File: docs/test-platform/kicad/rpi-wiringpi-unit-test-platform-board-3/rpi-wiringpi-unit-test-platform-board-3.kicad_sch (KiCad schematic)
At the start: 22 parts, among them J1 JST_IN_PWR, J2 JST_IN_SIG, J3 JST_OUT_PWR, J4 JST_OUT_SW, J5 JST_OUT_COIL, J6 JST_IO_A4_7, J7 JST_IO_B0_3, J8 JST_IO_B4_7, SW1 DIP_SW_x3, U1 MCP23017_0x20, U2 MCP23017_0x21

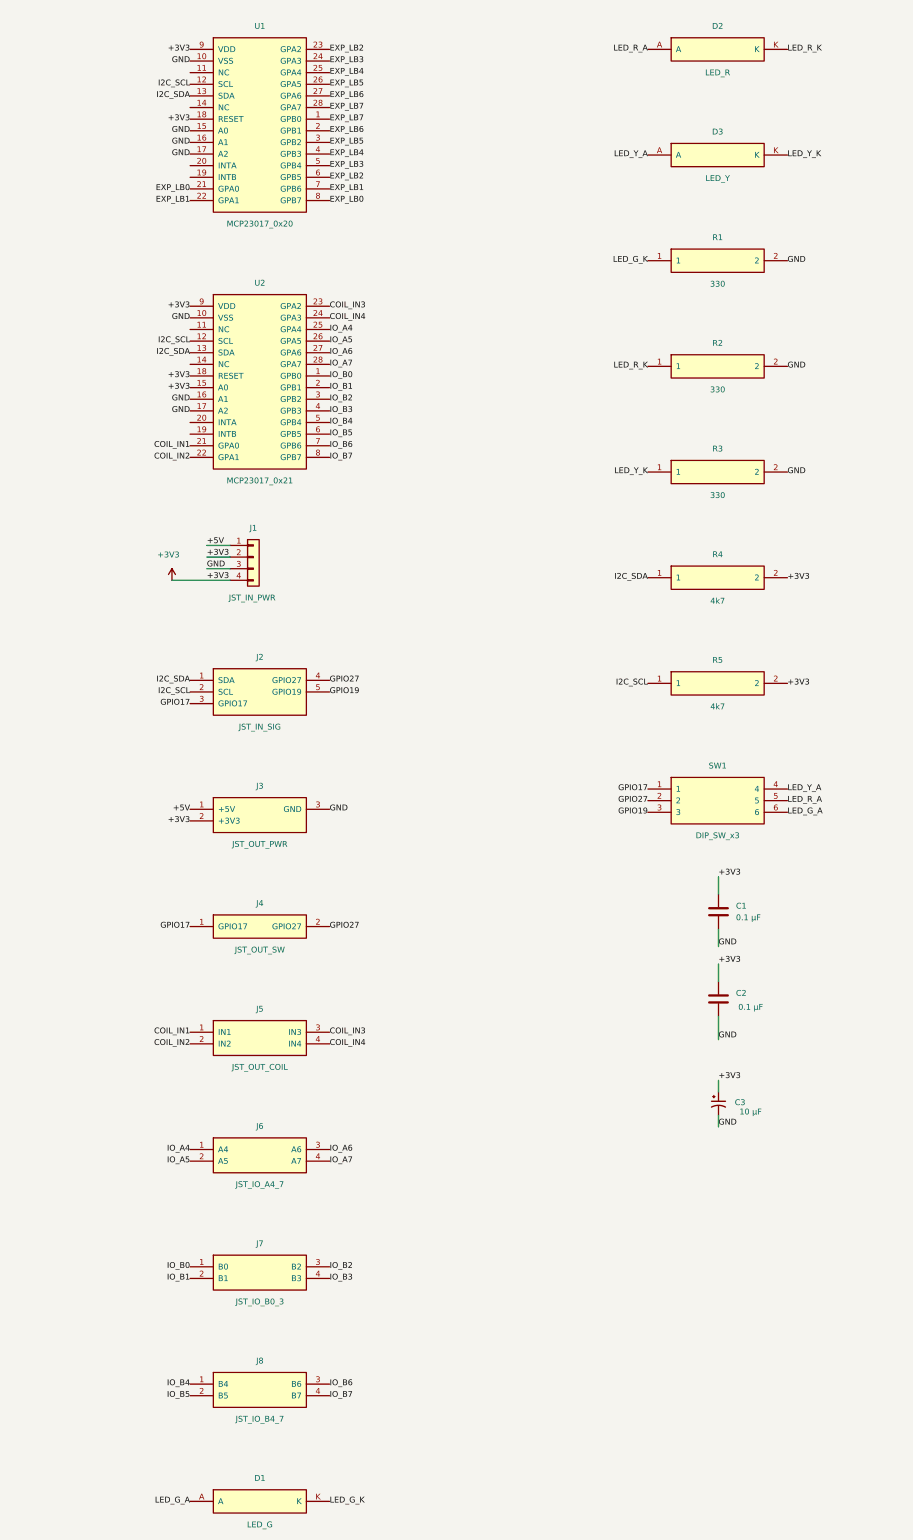
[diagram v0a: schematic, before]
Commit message: Updated boards
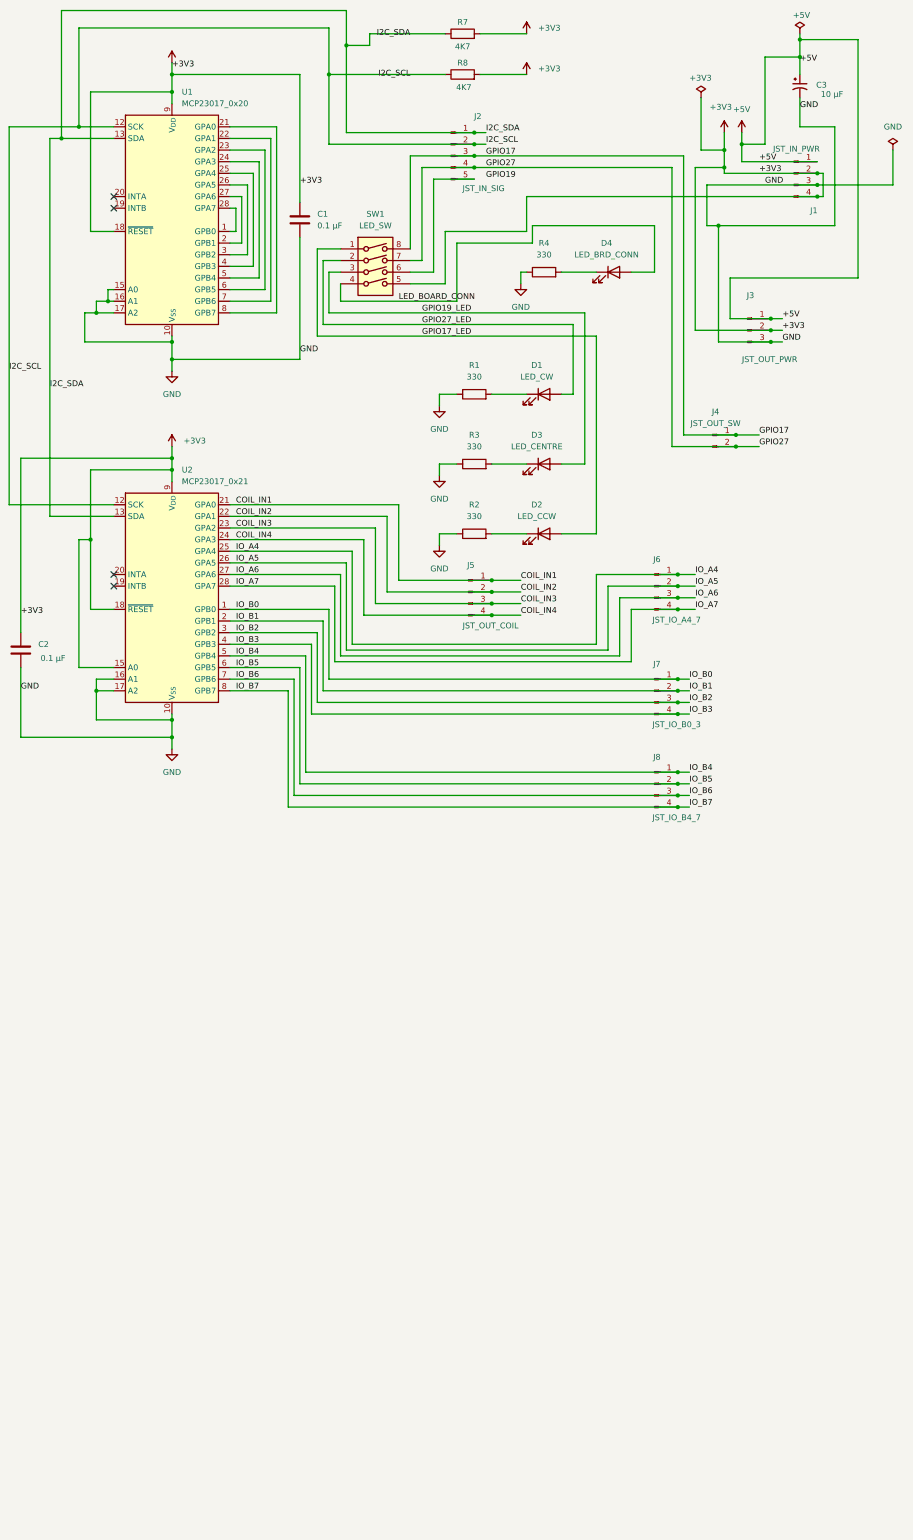
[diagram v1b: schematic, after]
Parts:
- removed D1: LED_G, rpi-wiringpi-unit-test-platform-board-3:D1, symbol rpi-wiringpi-unit-test-platform-board-3:D1
- removed D2: LED_R, rpi-wiringpi-unit-test-platform-board-3:D2, symbol rpi-wiringpi-unit-test-platform-board-3:D2
- removed D3: LED_Y, rpi-wiringpi-unit-test-platform-board-3:D3, symbol rpi-wiringpi-unit-test-platform-board-3:D3
- removed J1: JST_IN_PWR, rpi-wiringpi-unit-test-platform-board-3:J1, symbol Connector_Generic:Conn_01x04
- removed J2: JST_IN_SIG, rpi-wiringpi-unit-test-platform-board-3:J2, symbol rpi-wiringpi-unit-test-platform-board-3:J2
- removed J3: JST_OUT_PWR, rpi-wiringpi-unit-test-platform-board-3:J3, symbol rpi-wiringpi-unit-test-platform-board-3:J3
- removed J4: JST_OUT_SW, rpi-wiringpi-unit-test-platform-board-3:J4, symbol rpi-wiringpi-unit-test-platform-board-3:J4
- removed J5: JST_OUT_COIL, rpi-wiringpi-unit-test-platform-board-3:J5, symbol rpi-wiringpi-unit-test-platform-board-3:J5
- removed J6: JST_IO_A4_7, rpi-wiringpi-unit-test-platform-board-3:J6, symbol rpi-wiringpi-unit-test-platform-board-3:J6
- removed J7: JST_IO_B0_3, rpi-wiringpi-unit-test-platform-board-3:J7, symbol rpi-wiringpi-unit-test-platform-board-3:J7
- removed J8: JST_IO_B4_7, rpi-wiringpi-unit-test-platform-board-3:J8, symbol rpi-wiringpi-unit-test-platform-board-3:J8
- removed R1: 330, rpi-wiringpi-unit-test-platform-board-3:R1, symbol rpi-wiringpi-unit-test-platform-board-3:R1
- removed R2: 330, rpi-wiringpi-unit-test-platform-board-3:R2, symbol rpi-wiringpi-unit-test-platform-board-3:R2
- removed R3: 330, rpi-wiringpi-unit-test-platform-board-3:R3, symbol rpi-wiringpi-unit-test-platform-board-3:R3
- removed R4: 4k7, rpi-wiringpi-unit-test-platform-board-3:R4, symbol rpi-wiringpi-unit-test-platform-board-3:R4
- removed R5: 4k7, rpi-wiringpi-unit-test-platform-board-3:R5, symbol rpi-wiringpi-unit-test-platform-board-3:R5
- removed SW1: DIP_SW_x3, rpi-wiringpi-unit-test-platform-board-3:SW1, symbol rpi-wiringpi-unit-test-platform-board-3:SW1
- removed U1: MCP23017_0x20, rpi-wiringpi-unit-test-platform-board-3:U1, symbol rpi-wiringpi-unit-test-platform-board-3:U1
- removed U2: MCP23017_0x21, rpi-wiringpi-unit-test-platform-board-3:U2, symbol rpi-wiringpi-unit-test-platform-board-3:U2
- added D1: LED_CW, LED_THT:LED_D5.0mm, symbol Device:LED
- added D2: LED_CCW, LED_THT:LED_D5.0mm, symbol Device:LED
- added D3: LED_CENTRE, LED_THT:LED_D5.0mm, symbol Device:LED
- added D4: LED_BRD_CONN, LED_THT:LED_D5.0mm, symbol Device:LED
- added J1: JST_IN_PWR, Connector_JST:JST_XH_B4B-XH-A_1x04_P2.50mm_Vertical, symbol Connector:Conn_01x04_Pin
- added J2: JST_IN_SIG, Connector_JST:JST_XH_B5B-XH-A_1x05_P2.50mm_Vertical, symbol Connector:Conn_01x05_Pin
- added J3: JST_OUT_PWR, Connector_JST:JST_XH_B3B-XH-A_1x03_P2.50mm_Vertical, symbol Connector:Conn_01x03_Pin
- added J4: JST_OUT_SW, Connector_JST:JST_XH_B2B-XH-A_1x02_P2.50mm_Vertical, symbol Connector:Conn_01x02_Pin
- added J5: JST_OUT_COIL, Connector_JST:JST_XH_B4B-XH-A_1x04_P2.50mm_Vertical, symbol Connector:Conn_01x04_Pin
- added J6: JST_IO_A4_7, Connector_JST:JST_XH_B4B-XH-A_1x04_P2.50mm_Vertical, symbol Connector:Conn_01x04_Pin
- added J7: JST_IO_B0_3, Connector_JST:JST_XH_B4B-XH-A_1x04_P2.50mm_Vertical, symbol Connector:Conn_01x04_Pin
- added J8: JST_IO_B4_7, Connector_JST:JST_XH_B4B-XH-A_1x04_P2.50mm_Vertical, symbol Connector:Conn_01x04_Pin
- added R1, R2, R3, R4: 330, Resistor_THT:R_Axial_DIN0207_L6.3mm_D2.5mm_P7.62mm_Horizontal, symbol Device:R
- added R7, R8: 4K7, Resistor_THT:R_Axial_DIN0207_L6.3mm_D2.5mm_P7.62mm_Horizontal, symbol Device:R
- added SW1: LED_SW, Button_Switch_THT:SW_DIP_SPSTx04_Slide_6.7x11.72mm_W7.62mm_P2.54mm_LowProfile, symbol Switch:SW_DIP_x04
- added U1: MCP23017_0x20, Package_DIP:DIP-28_W7.62mm, symbol Interface_Expansion:MCP23017x-x-SP
- added U2: MCP23017_0x21, Package_DIP:DIP-28_W7.62mm, symbol Interface_Expansion:MCP23017x-x-SP
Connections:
- net +3V3: now also J1.2 (Pin_2), J1.4 (Pin_4), J3.2 (Pin_2), R7.2, R8.2, SW1.5, U1.18 (~{RESET}), U1.9 (V_{DD}), U2.15 (A0), U2.18 (~{RESET}), U2.9 (V_{DD}); no longer C3.1
- net +5V: now also C3.1, J1.1 (Pin_1), J3.1 (Pin_1)
- net COIL_IN1: now also J5.1 (Pin_1), U2.21 (GPA0)
- net COIL_IN2: now also J5.2 (Pin_2), U2.22 (GPA1)
- net COIL_IN3: now also J5.3 (Pin_3), U2.23 (GPA2)
- net COIL_IN4: now also J5.4 (Pin_4), U2.24 (GPA3)
- net GND: now also J1.3 (Pin_3), J3.3 (Pin_3), R1.1, R2.1, R3.1, R4.1, U1.10 (V_{SS}), U1.15 (A0), U1.16 (A1), U1.17 (A2), U2.10 (V_{SS}), U2.16 (A1), U2.17 (A2)
- net GPIO17: now also J2.3 (Pin_3), J4.1 (Pin_1), SW1.8
- net GPIO27: now also J2.4 (Pin_4), J4.2 (Pin_2), SW1.7
- net I2C_SCL: now also J2.2 (Pin_2), R8.1, U1.12 (SCK), U2.12 (SCK)
- net I2C_SDA: now also J2.1 (Pin_1), R7.1, U1.13 (SDA), U2.13 (SDA)
- net IO_A4: now also J6.1 (Pin_1), U2.25 (GPA4)
- net IO_A5: now also J6.2 (Pin_2), U2.26 (GPA5)
- net IO_A6: now also J6.3 (Pin_3), U2.27 (GPA6)
- net IO_A7: now also J6.4 (Pin_4), U2.28 (GPA7)
- net IO_B0: now also J7.1 (Pin_1), U2.1 (GPB0)
- net IO_B1: now also J7.2 (Pin_2), U2.2 (GPB1)
- net IO_B2: now also J7.3 (Pin_3), U2.3 (GPB2)
- net IO_B3: now also J7.4 (Pin_4), U2.4 (GPB3)
- net IO_B4: now also J8.1 (Pin_1), U2.5 (GPB4)
- net IO_B5: now also J8.2 (Pin_2), U2.6 (GPB5)
- net IO_B6: now also J8.3 (Pin_3), U2.7 (GPB6)
- net IO_B7: now also J8.4 (Pin_4), U2.8 (GPB7)
- new net: D4.1 (K), R4.2
- new net: J2.5 (Pin_5), SW1.6
- new net: D3.1 (K), R3.2
- new net: D2.1 (K), R2.2
- new net: U1.1 (GPB0), U1.28 (GPA7)
- new net: U1.2 (GPB1), U1.27 (GPA6)
- new net: U1.21 (GPA0), U1.8 (GPB7)
- new net: U1.22 (GPA1), U1.7 (GPB6)
- new net: U1.23 (GPA2), U1.6 (GPB5)
- new net: U1.24 (GPA3), U1.5 (GPB4)
- new net: U1.25 (GPA4), U1.4 (GPB3)
- new net: U1.26 (GPA5), U1.3 (GPB2)
- new net: D1.1 (K), R1.2
- new net GPIO17_LED: D2.2 (A), SW1.1
- new net GPIO19_LED: D3.2 (A), SW1.3
- new net GPIO27_LED: D1.2 (A), SW1.2
- new net LED_BOARD_CONN: D4.2 (A), SW1.4
- no-connect marks 0 -> 4
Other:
- moved on the sheet: C1, C2, C3
